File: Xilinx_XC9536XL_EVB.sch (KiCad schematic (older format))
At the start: 54 parts, among them IC1 ATTINY2313-P, P1 CONN_7X2, P2 CONN_2, P3 CONN_3X2, P4 CONN_5, P5 CONN_5, P6 CONN_12, P7 CONN_6, P8 CONN_8, SW1 SW_PUSH, SW2 SW_DIP_8, U1 XC9536XLPC44, X1 XTAL

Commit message: updated footprints libraries (pull-request to official git pending)
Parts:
- C1, C2, C3, C5, C6: footprint (none) -> Capacitors_ThroughHole:C_Rect_L7_W2_P5
- C4: footprint (none) -> Capacitors_ThroughHole:C_Radial_D5_L6_P2.5
- C7, C8: footprint (none) -> Capacitors_ThroughHole:C_Rect_L4_W2.5_P2.5
- D1, D2, D3, D4, D5, D6, D7, D8: footprint (none) -> LEDs:LED-3MM
- IC1: footprint DIL20 -> Sockets_DIP:DIP-20__300; symbol ATTINY2313-P_OLD -> ATTINY2313-P_old
- P1: footprint (none) -> Connect_custom:IDC_Header_Straight_14pins
- P2: footprint (none) -> Connect:bornier2
- P3: footprint (none) -> Pin_Headers:Pin_Header_Straight_2x03
- P4, P5: footprint (none) -> Pin_Headers:Pin_Header_Straight_1x05
- P6: footprint (none) -> Pin_Headers:Pin_Header_Straight_1x12
- P7: footprint (none) -> Pin_Headers:Pin_Header_Straight_1x06
- P8: footprint (none) -> Pin_Headers:Pin_Header_Straight_1x08
- R1, R10, R11, R12, R13, R14, R15, R16, R17, R18, R19, R2, R20, R21, R22, R23, R24, R3, R4, R5, R6, R7, R8, R9: footprint (none) -> Resistors_ThroughHole_custom:Resistor_Horizontal_RM7mm
- RR1: footprint (none) -> Resistors_ThroughHole_custom:Resistor_Array_SIP8
- SW1: footprint (none) -> Buttons_Switches_ThroughHole:SW_PUSH_SMALL
- SW2: footprint (none) -> Buttons_Switches_ThroughHole:SW_DIP_x8_Slide
- U1: footprint (none) -> Sockets:PLCC44
- X1: footprint (none) -> Crystals:Crystal_HC48-U_Vertical

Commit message: updated pcb with new footprints + removed old files
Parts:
- X1: footprint Crystals:Crystal_HC48-U_Vertical -> Crystals:Crystal_HC49-U_Vertical
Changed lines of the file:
@@
 EESchema Schematic File Version 2
-LIBS:Xilinx_XC9536XL_EVB-rescue
 LIBS:power
 LIBS:device
@@
 F 0 "X1" H 2375 3500 60  0000 C CNN
 F 1 "XTAL" H 2300 3200 60  0001 C CNN
-F 2 "Crystals:Crystal_HC48-U_Vertical" H 2200 3350 60  0001 C CNN
+F 2 "Crystals:Crystal_HC49-U_Vertical" H 2200 3350 60  0001 C CNN
 F 3 "" H 2200 3350 60  0001 C CNN
 	1    2200 3350

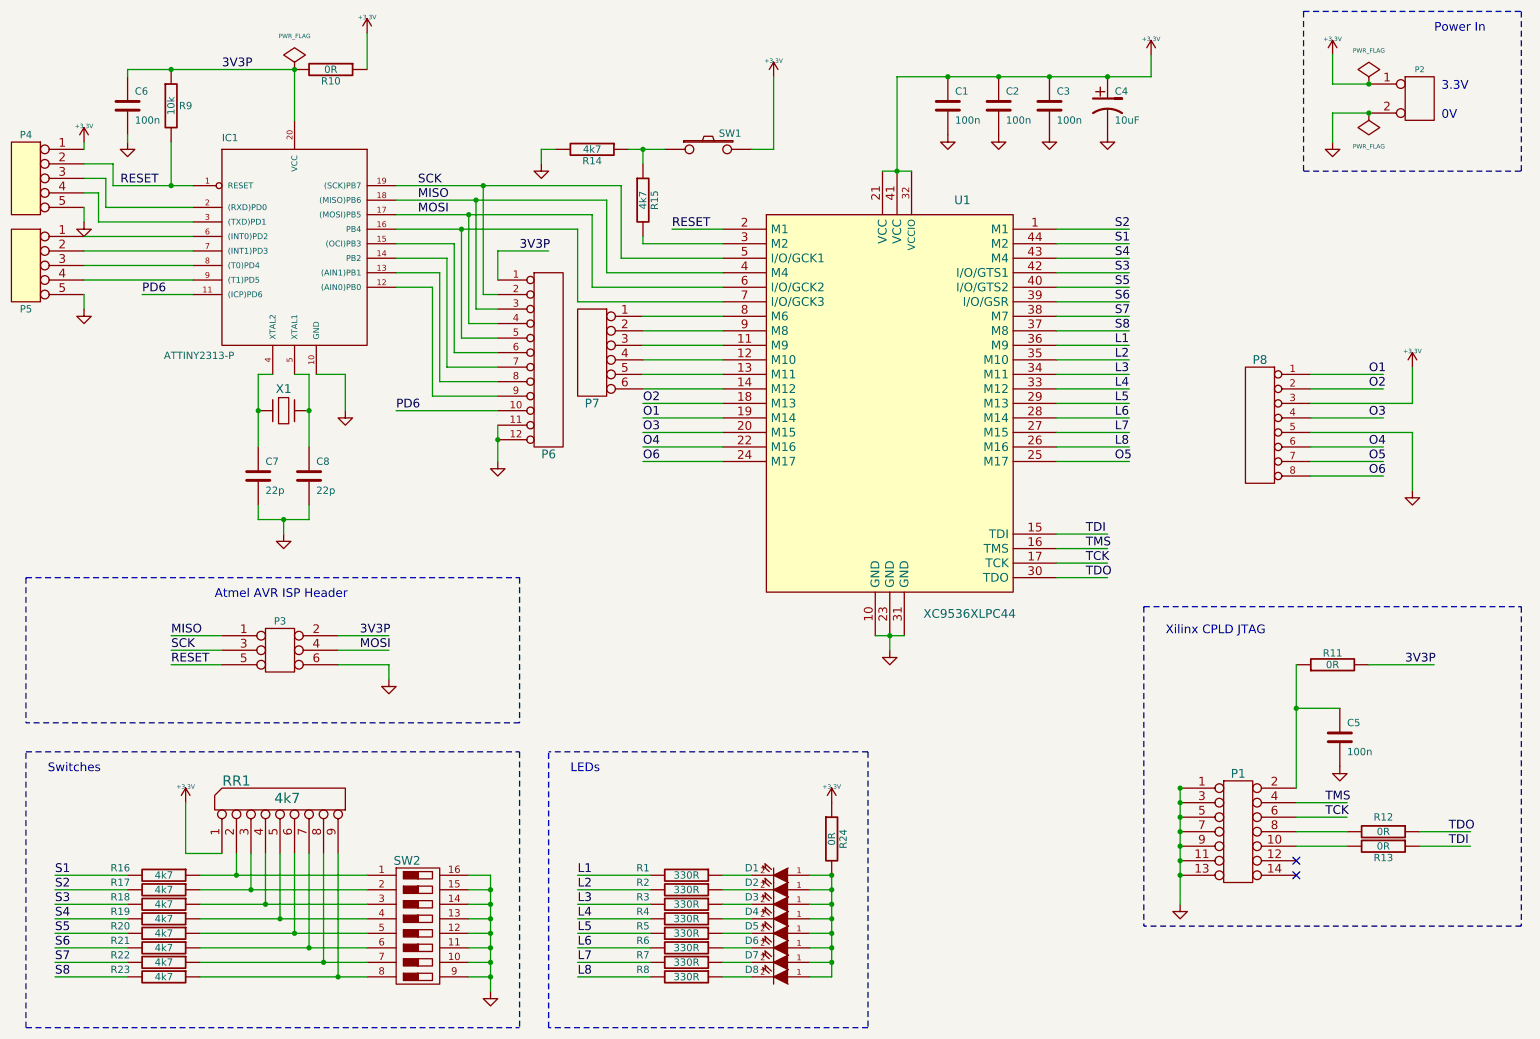
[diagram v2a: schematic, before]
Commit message: even more clean up
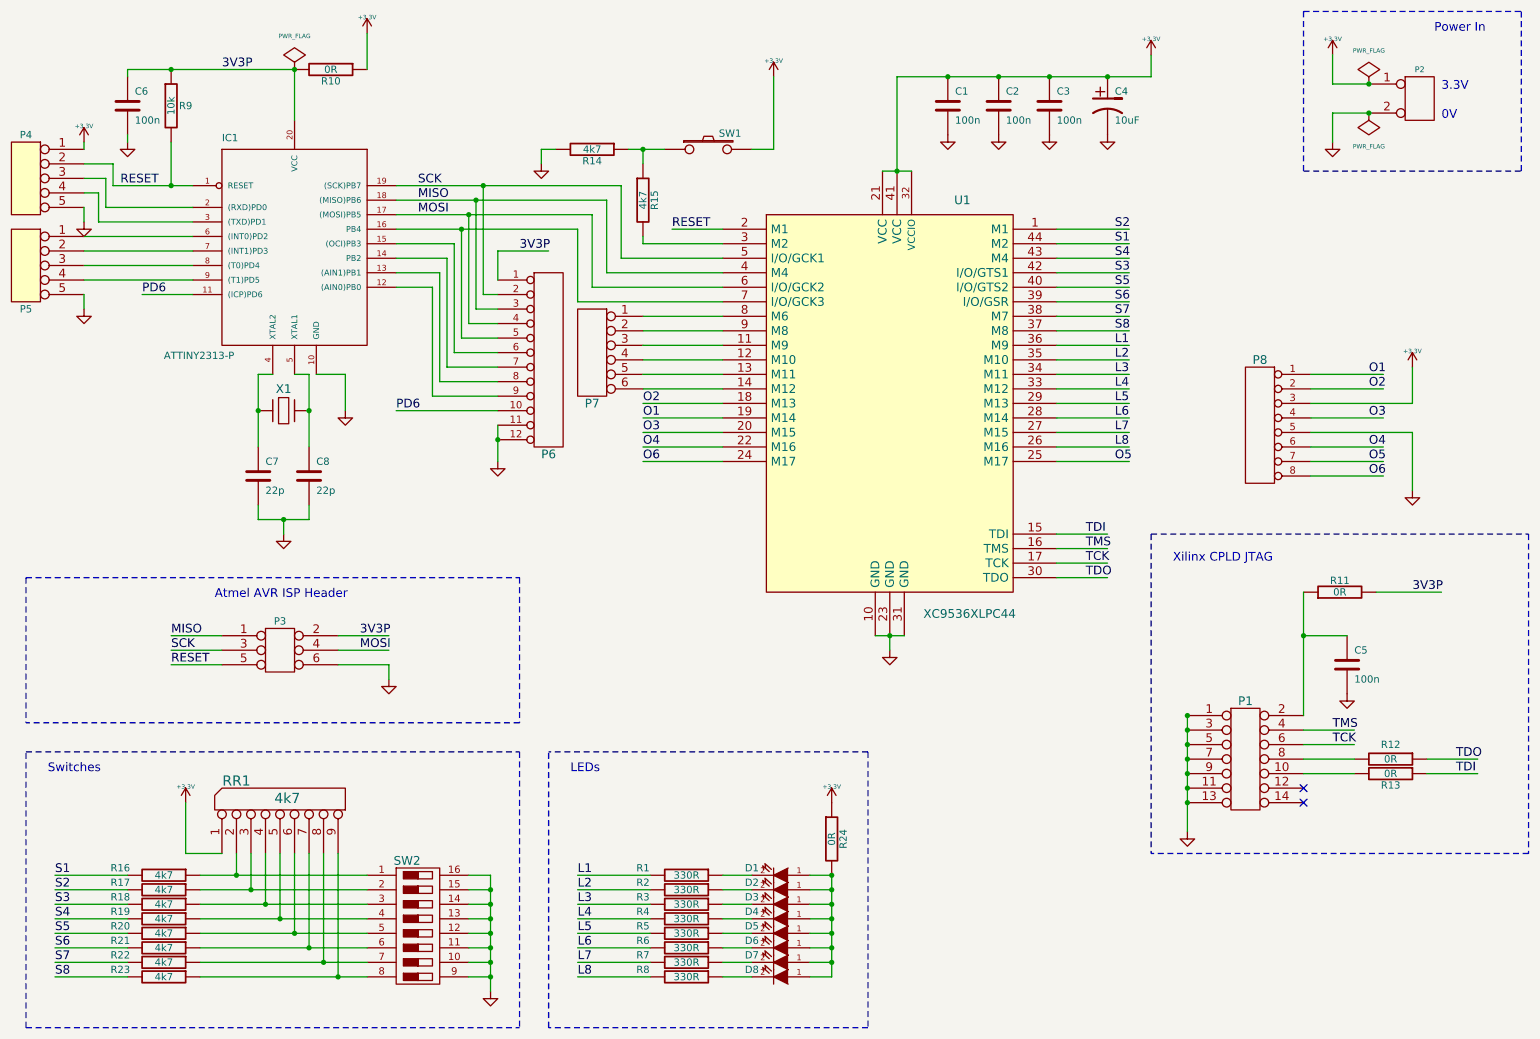
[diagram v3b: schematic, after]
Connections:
- wire segments 207 -> 252
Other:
- moved on the sheet: C5, P1, R11, R12, R13
